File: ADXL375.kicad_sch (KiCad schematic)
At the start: 5 parts, among them U9 ADXL372BCCZ-RL

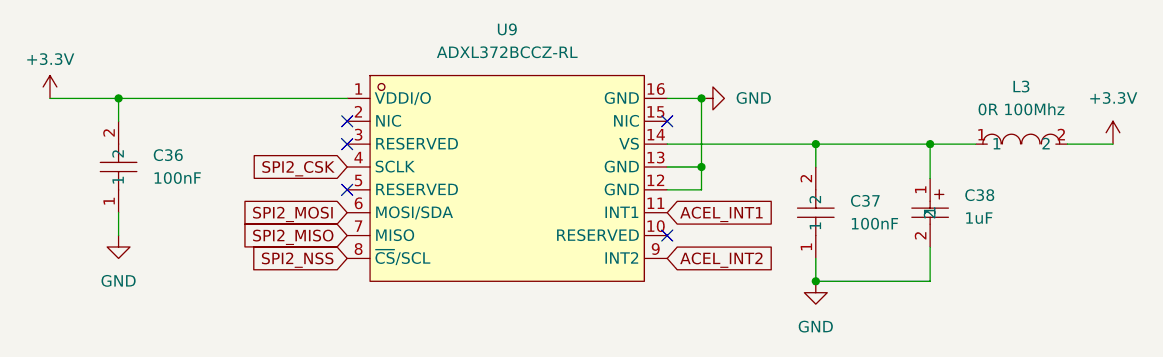
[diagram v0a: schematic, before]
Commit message: Todo antes de PCB
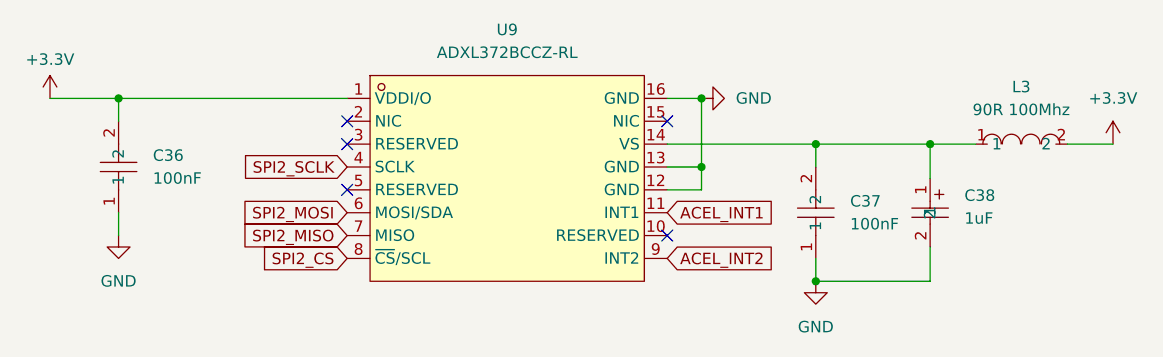
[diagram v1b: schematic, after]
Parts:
- L3: value 0R 100Mhz -> 90R 100Mhz; footprint Inductor_SMD:L_0402_1005Metric_Pad0.77x0.64mm_HandSolder -> Inductor_SMD:L_0603_1608Metric_Pad1.05x0.95mm_HandSolder; LCSC Part C139137 -> C50325905; MPN CBG100505U000T -> APBD1608-900WTD12
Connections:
- net SPI2_CSK renamed SPI2_SCLK
- net SPI2_NSS renamed SPI2_CS
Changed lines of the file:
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@@
 		)
 	)
-	(global_label "SPI2_NSS"
+	(global_label "SPI2_CS"
 		(shape input)
 		(at 153.67 106.68 180)
@@
 		)
 		(property "Intersheetrefs" "${INTERSHEET_REFS}"
-			(at 141.6739 106.68 0)
+			(at 142.9439 106.68 0)
 			(hide yes)
 			(show_name no)
@@
 		)
 	)
-	(global_label "SPI2_CSK"
+	(global_label "SPI2_SCLK"
 		(shape input)
 		(at 153.67 96.52 180)
@@
 		)
 		(property "Intersheetrefs" "${INTERSHEET_REFS}"
-			(at 141.6739 96.52 0)
+			(at 140.6458 96.52 0)
 			(hide yes)
 			(show_name no)
@@
 			)
 		)
-		(property "Value" "0R 100Mhz"
+		(property "Value" "90R 100Mhz"
 			(at 228.57 90.17 0)
 			(show_name no)
@@
 			)
 		)
-		(property "Footprint" "Inductor_SMD:L_0402_1005Metric_Pad0.77x0.64mm_HandSolder"
+		(property "Footprint" "Inductor_SMD:L_0603_1608Metric_Pad1.05x0.95mm_HandSolder"
 			(at 228.6 101.6 0)
 			(hide yes)
@@
 			)
 		)
-		(property "Datasheet" "https://lcsc.com/product-detail/Ferrite-Beads-And-Chips_0R-25_C139137.html"
+		(property "Datasheet" "https://www.lcsc.com/datasheet/C50325905.pdf?spm=wm.sxq.inf.ggs___wm.fly.bg.2.xh&lcsc_vid=E1NWVQUCRlhbBlQCFAQIVQJXQ1UKV1AATgdWXgAERFExVlNeRVBaX1ZST1RWXjsOAxUeFF5JWBYZEEoKFBINSQcJGk4dAgUUFAk%3D"
 			(at 228.6 104.14 0)
 			(hide yes)
@@
 			)
 		)
-		(property "MPN" "CBG100505U000T"
+		(property "MPN" "APBD1608-900WTD12"
 			(at 228.6 109.22 0)
 			(hide yes)
@@
 			)
 		)
-		(property "LCSC Part" "C139137"
+		(property "LCSC Part" "C50325905"
 			(at 228.6 111.76 0)
 			(hide yes)
